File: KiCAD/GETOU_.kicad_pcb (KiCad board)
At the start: 2 copper layers, 119.5 x 61 mm, 25 parts, among them U1 XIAO-RP2040-DIP

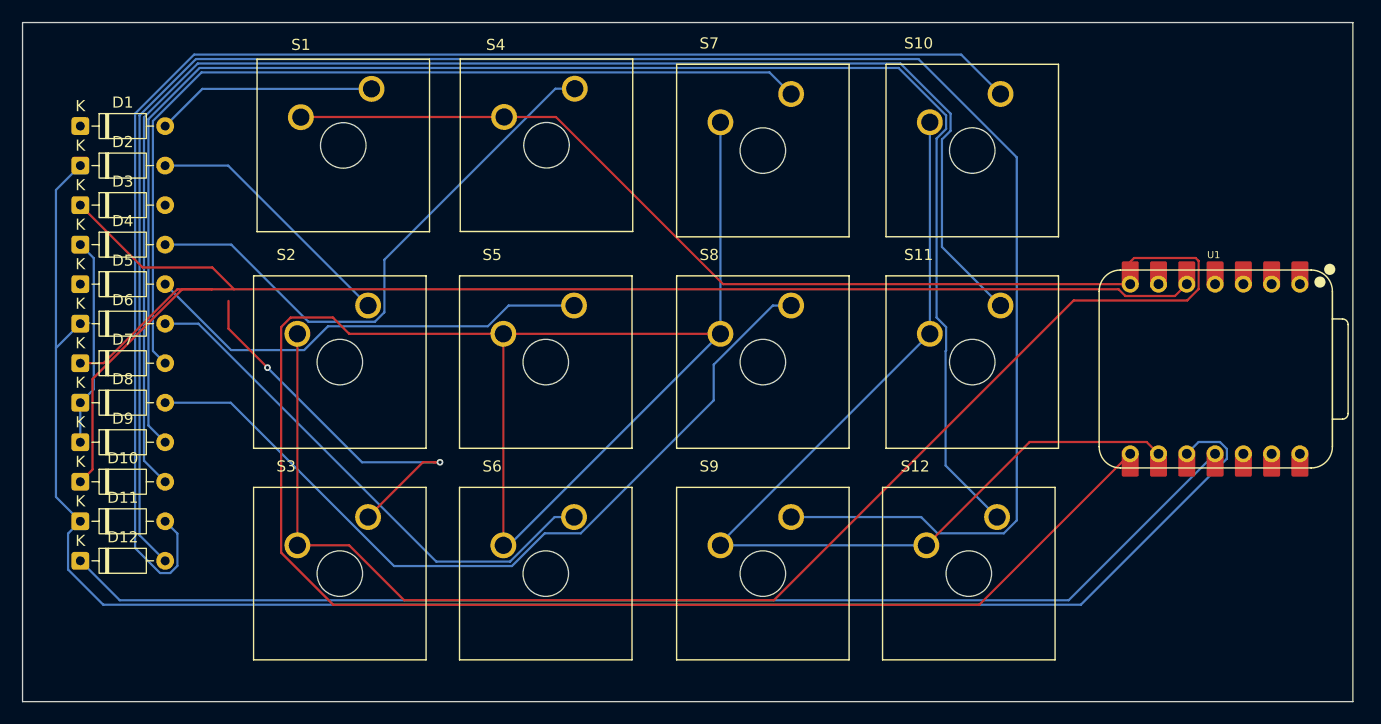
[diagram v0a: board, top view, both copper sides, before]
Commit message: Modify Files
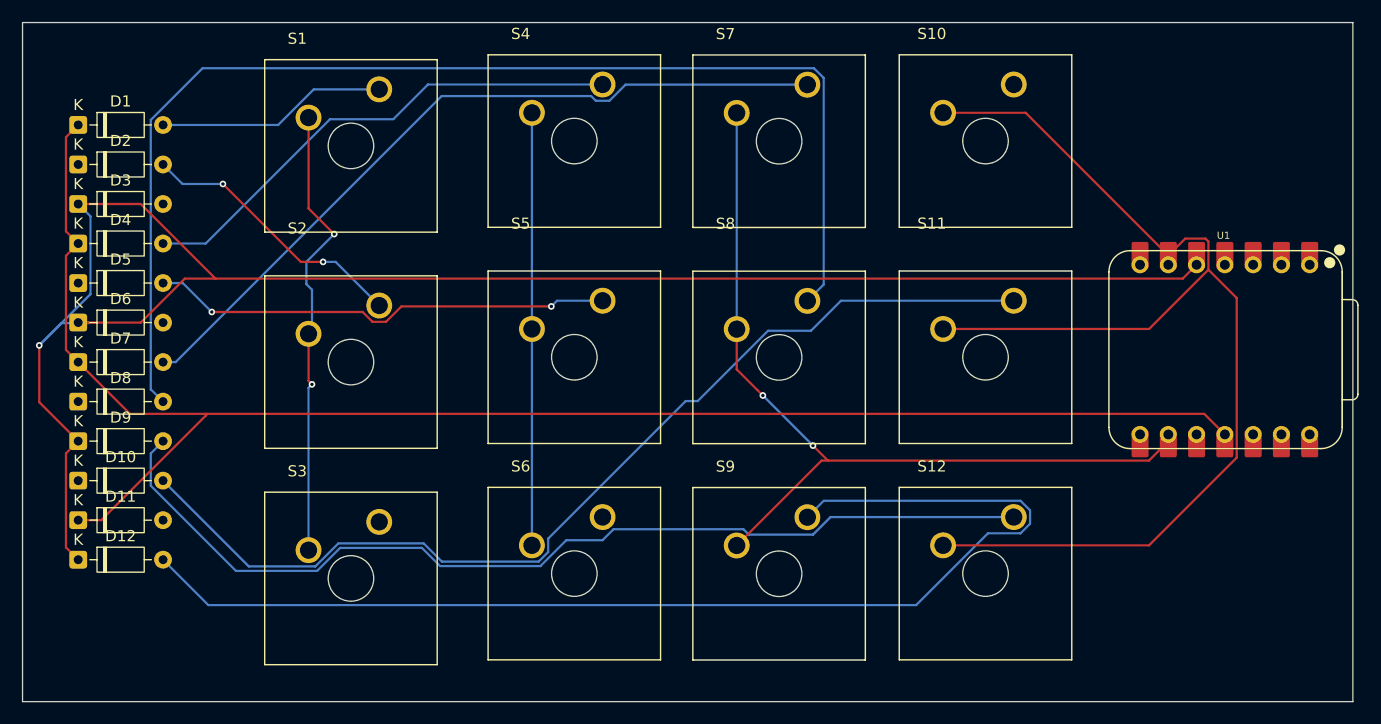
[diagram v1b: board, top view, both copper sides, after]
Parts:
- moved S5 2.60 mm to (142.1, 90.6)
- moved S6 2.57 mm to (142.1, 110.0)
- moved S4 2.53 mm to (142.1, 71.1)
- moved U1 1.95 mm to (200.5, 89.9)
- moved S7 1.68 mm to (160.5, 71.2)
- moved S8 1.52 mm to (160.5, 90.6)
- moved S12 1.50 mm to (179.0, 110.0)
- moved S10 1.46 mm to (179.0, 71.1)
- moved S9 1.46 mm to (160.5, 110.0)
- moved S11 1.27 mm to (179.0, 90.6)
- moved S3 1.09 mm to (122.0, 110.4)
- moved S2 1.00 mm to (122.0, 91.0)
- moved S1 0.69 mm to (122.0, 71.6)
- moved D3 0.21 mm to (97.5, 76.8)
- moved D4 0.21 mm to (97.5, 80.3)
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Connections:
- D10 pad 1: col2 -> col1
- D11 pad 1: col1 -> col0
- D12 pad 1: col0 -> col2
- D4 pad 1: col3 -> col0
- D5 pad 1: col0 -> col1
- D6 pad 1: col1 -> col2
- D7 pad 1: col2 -> col0
- D8 pad 1: col3 -> col1
- D9 pad 1: col3 -> col2
- S10 pad 1: row2 -> row3
- S11 pad 1: row2 -> row3
- S12 pad 1: row2 -> row3
- S4 pad 1: row0 -> row1
- S7 pad 1: row1 -> row2
- S8 pad 1: row1 -> row2
- U1 pad 6: col3 -> row3
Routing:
- net row1: track 209.9 -> 38.9 mm
- net row0: track 205.2 -> 41.4 mm, vias 0 -> 2
- net col1: track 159.4 -> 0.00 mm
- net Net-(D11-A): track 129.9 -> 0.00 mm
- net row3: track 0.00 -> 106.0 mm
- net Net-(D12-A): track 179.5 -> 104.8 mm
- net Net-(D9-A): track 143.7 -> 88.9 mm
- net Net-(D6-A): track 47.2 -> 0.00 mm
- net Net-(D10-A): track 129.6 -> 91.6 mm
- net col0: track 108.8 -> 144.3 mm
- net Net-(D3-A): track 35.5 -> 0.00 mm, vias 2 -> 0
- net Net-(D8-A): track 73.9 -> 109.1 mm
- net col3: track 18.8 -> 0.00 mm
- net col2: track 143.5 -> 160.7 mm, vias 0 -> 1
- net Net-(D7-A): track 82.2 -> 68.6 mm
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
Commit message: Modifiy Files
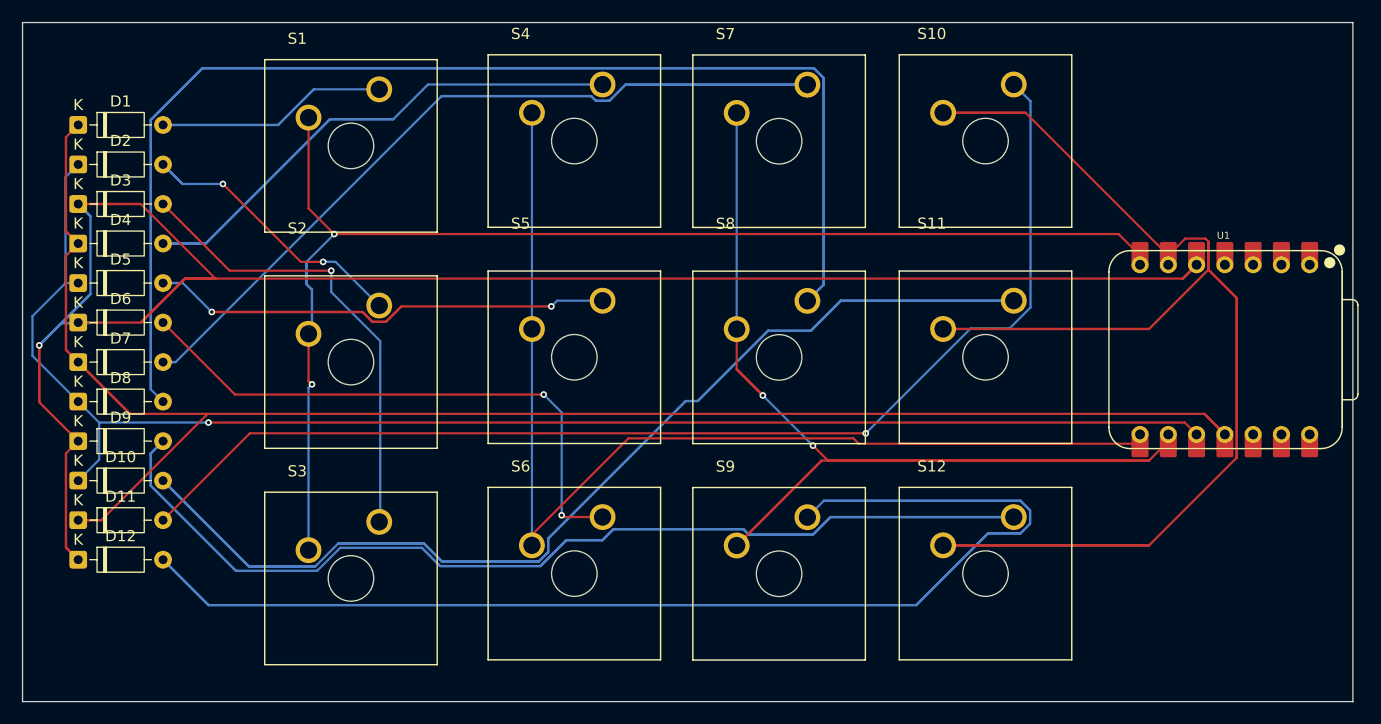
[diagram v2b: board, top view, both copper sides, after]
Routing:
- net col1: track 0.00 -> 134.4 mm, vias 0 -> 1
- net Net-(D8-A): track 109.1 -> 216.7 mm
- net Net-(D11-A): track 0.00 -> 106.5 mm, vias 0 -> 1
- net Net-(D12-A): track 104.8 -> 207.5 mm
- net Net-(D10-A): track 91.6 -> 180.2 mm
- net Net-(D9-A): track 88.9 -> 174.9 mm
- net row0: track 41.4 -> 122.7 mm
- net row3: track 106.0 -> 171.7 mm
- net row1: track 38.9 -> 99.0 mm
- net Net-(D6-A): track 0.00 -> 52.1 mm, vias 0 -> 2
- net col2: track 160.7 -> 206.7 mm
- net row2: track 77.9 -> 121.4 mm
- net Net-(D3-A): track 0.00 -> 42.0 mm, vias 0 -> 1
- net Net-(D7-A): track 68.6 -> 103.3 mm
- net col0: track 144.3 -> 176.5 mm
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
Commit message: Modify Files
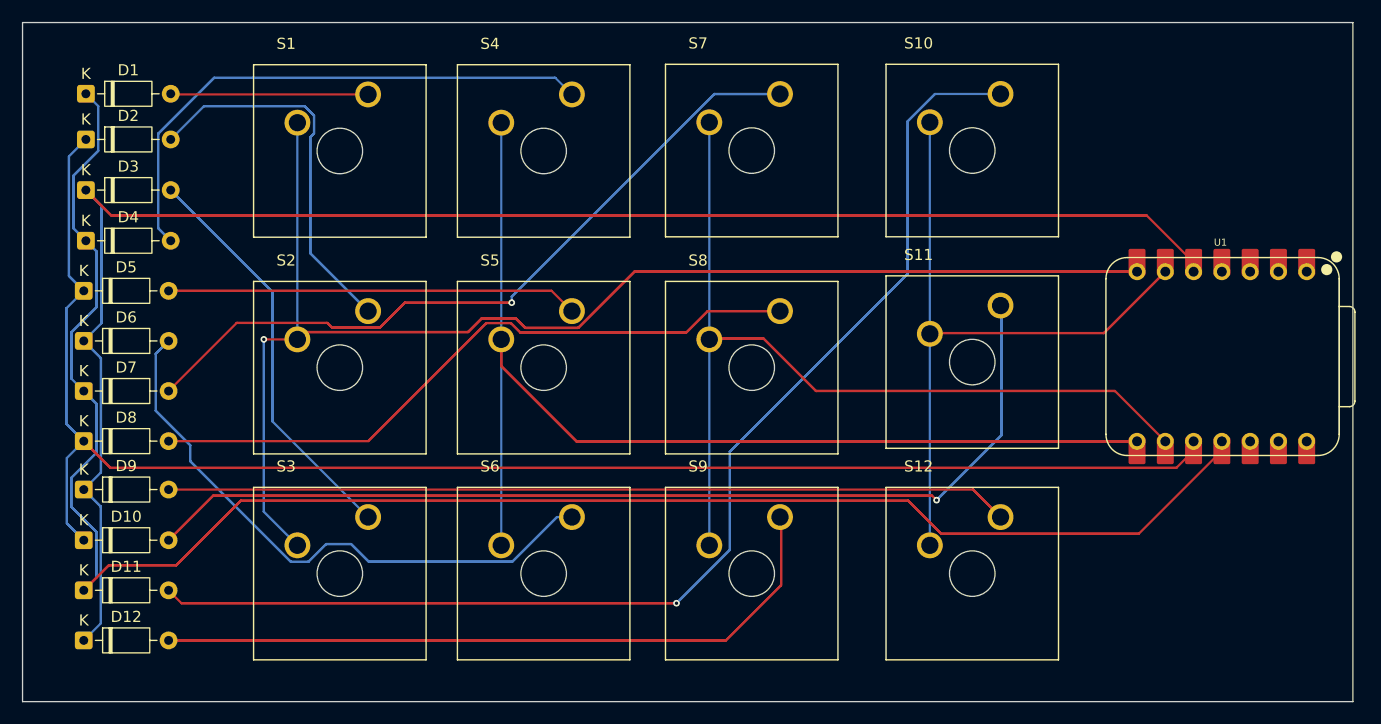
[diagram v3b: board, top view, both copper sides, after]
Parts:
- moved D12 7.27 mm to (98.0, 116.0)
- moved D11 6.32 mm to (98.0, 111.5)
- moved D10 5.37 mm to (98.0, 107.0)
- moved D9 4.38 mm to (98.0, 102.5)
- moved D8 3.59 mm to (98.0, 98.1)
- moved S5 2.91 mm to (139.3, 91.5)
- moved S4 2.90 mm to (139.3, 72.0)
- moved D1 2.88 mm to (98.2, 66.9)
- moved S6 2.76 mm to (139.3, 110.0)
- moved D7 2.65 mm to (98.0, 93.6)
- moved S8 2.63 mm to (158.0, 91.5)
- moved S7 2.60 mm to (158.0, 72.0)
- moved S9 2.46 mm to (158.0, 110.0)
- moved D2 2.35 mm to (98.2, 71.0)
- moved D6 1.72 mm to (98.0, 89.1)
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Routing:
- net row0: track 122.7 -> 293.5 mm, vias 2 -> 1
- net col1: track 134.4 -> 275.1 mm, vias 1 -> 0
- net col0: track 176.5 -> 308.2 mm
- net row1: track 99.0 -> 223.3 mm
- net Net-(D8-A): track 216.7 -> 103.0 mm
- net Net-(D11-A): track 106.5 -> 207.2 mm
- net Net-(D9-A): track 174.9 -> 79.2 mm
- net row3: track 171.7 -> 86.6 mm
- net Net-(D12-A): track 207.5 -> 126.3 mm
- net col2: track 206.7 -> 282.0 mm, vias 1 -> 0
- net Net-(D6-A): track 52.1 -> 105.8 mm, vias 2 -> 0
- net Net-(D2-A): track 28.4 -> 64.4 mm, vias 2 -> 0
- net Net-(D4-A): track 70.7 -> 97.8 mm
- net Net-(D7-A): track 103.3 -> 124.1 mm, vias 0 -> 1
- net Net-(D3-A): track 42.0 -> 61.3 mm, vias 1 -> 0
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
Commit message: Modify Files
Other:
- board text added: "getou_ Made by Kaihang(gnahiak2)"
